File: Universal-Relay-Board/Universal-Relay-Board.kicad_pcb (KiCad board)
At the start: 2 copper layers, 20.3 x 33.7 mm, 8 parts, among them J1 Conn_01x03_Male, J2 Screw_Terminal_01x03, K1 SRD-XXVDC-SL-C, Q1 2N7002

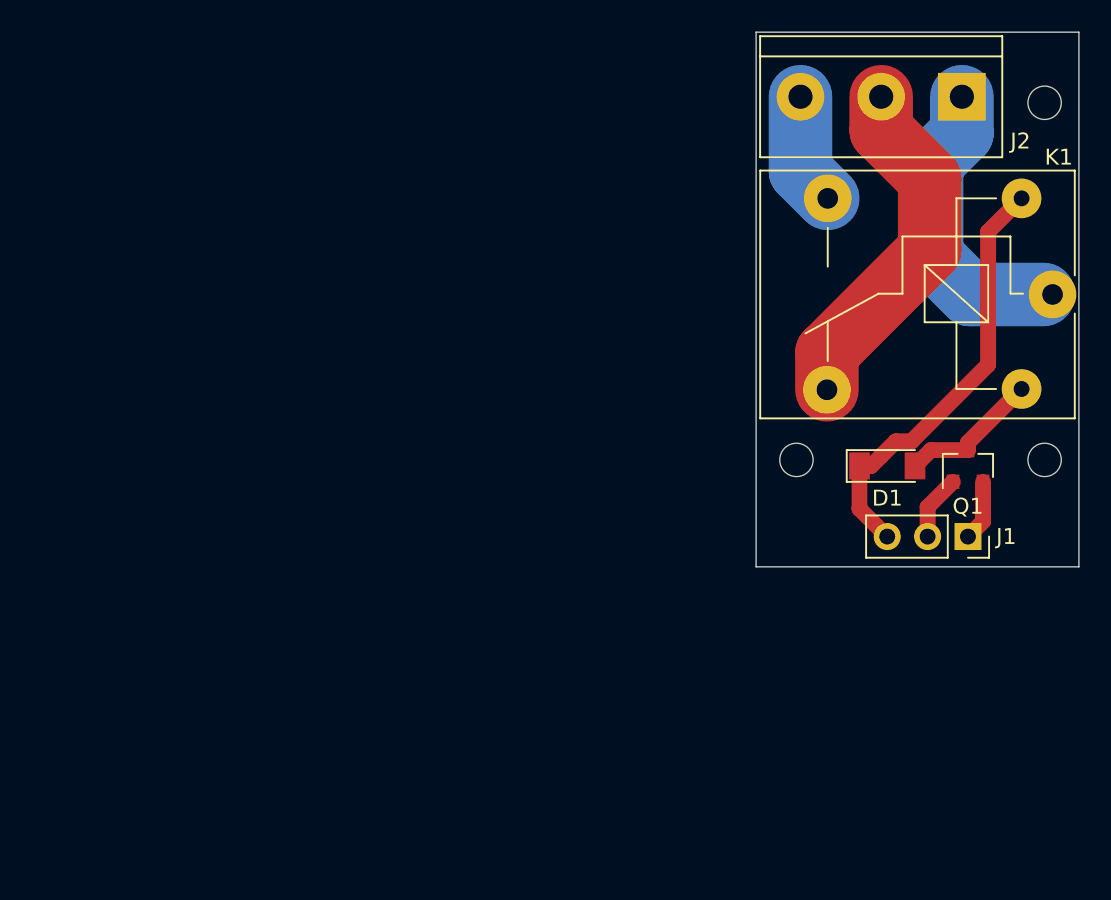
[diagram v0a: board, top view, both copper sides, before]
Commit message: multi channel done
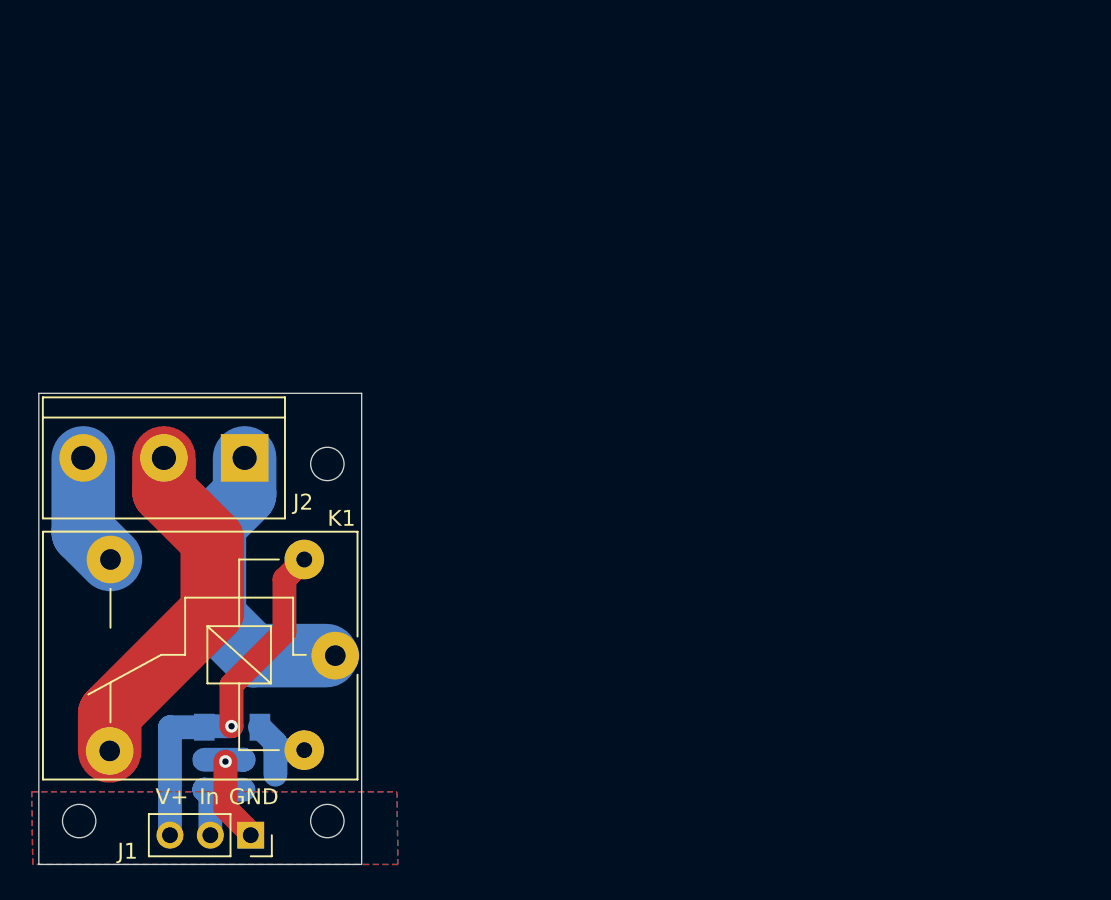
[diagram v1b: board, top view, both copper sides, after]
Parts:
- added R1: 10K, Resistor_SMD:R_0805_2012Metric, B.Cu at (74.5, 89.9)
- D1, Q1: moved to B.Cu
- moved J2 50.5 mm to (77.0, 70.0)
- moved H1 50.5 mm to (66.6, 92.8)
- moved H2 50.5 mm to (82.2, 70.4)
- moved H3 50.5 mm to (82.2, 92.8)
- moved K1 50.5 mm to (82.7, 82.4)
- moved J1 48.9 mm to (77.4, 93.7)
- moved Q1 48.6 mm to (78.0, 89.9), turned to 0 degrees
- moved D1 44.4 mm to (76.2, 86.9)
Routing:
- net VDD: track 27.3 -> 23.1 mm, vias 0 -> 1
- net GND: track 3.84 -> 7.77 mm, vias 0 -> 1
- net /CH1/Relay_Magnet_B: track 8.99 -> 5.65 mm
- net Net-(J1-Pad2): track 4.10 -> 5.51 mm
- added copper zone on F.Cu, net GND
- added copper zone on B.Cu, net VDD
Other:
- board size 20.3 x 33.7 mm -> 20.3 x 29.7 mm
- board text added: "22.35mm"
- board text added: "COM"
- board text added: "GND"
- board text added: "In"
- board text added: "NC"
- board text added: "NO"
- board text added: "V+"
